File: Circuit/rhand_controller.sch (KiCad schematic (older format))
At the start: 25 parts, among them P1 RU_ADC, P11 RW_ADC, P2 LU_ADC, P3 RV_ADC, P4 LV_ADC, P5 RW_ADC, P6 LW_ADC, P7 BLUETOOTH, P9 LW_ADC, SW1 EmSW, SW2 SWITCH_INV, U1 STM32F042, U2 IM315TX

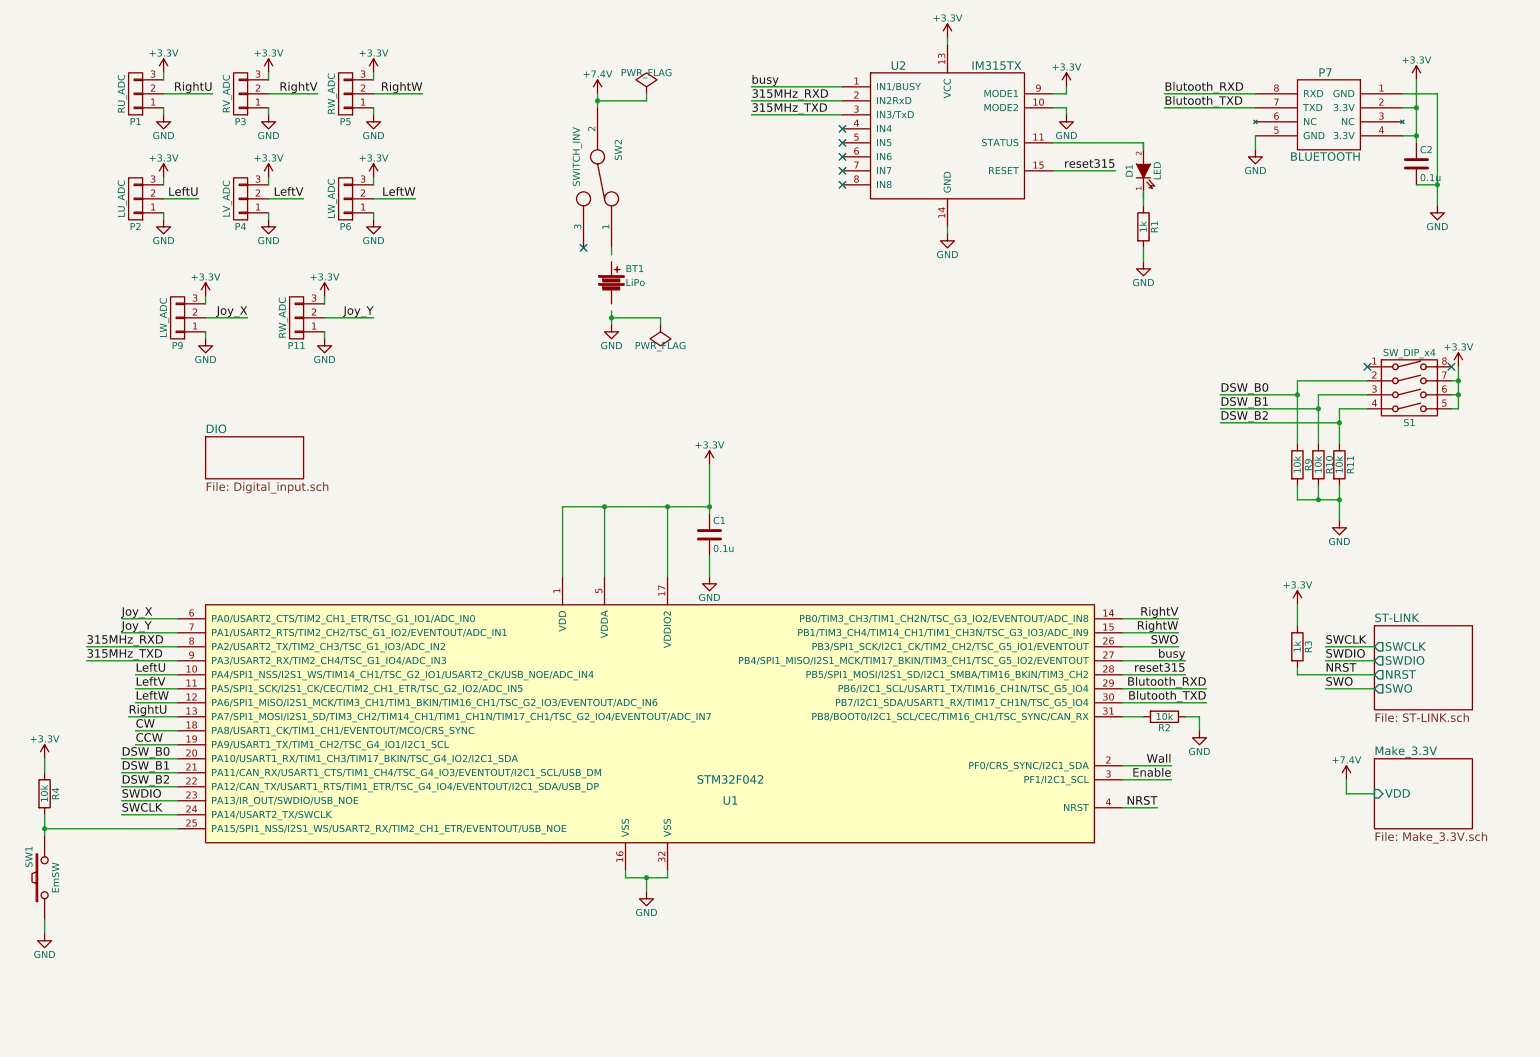
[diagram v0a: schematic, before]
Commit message: シート分けと移動
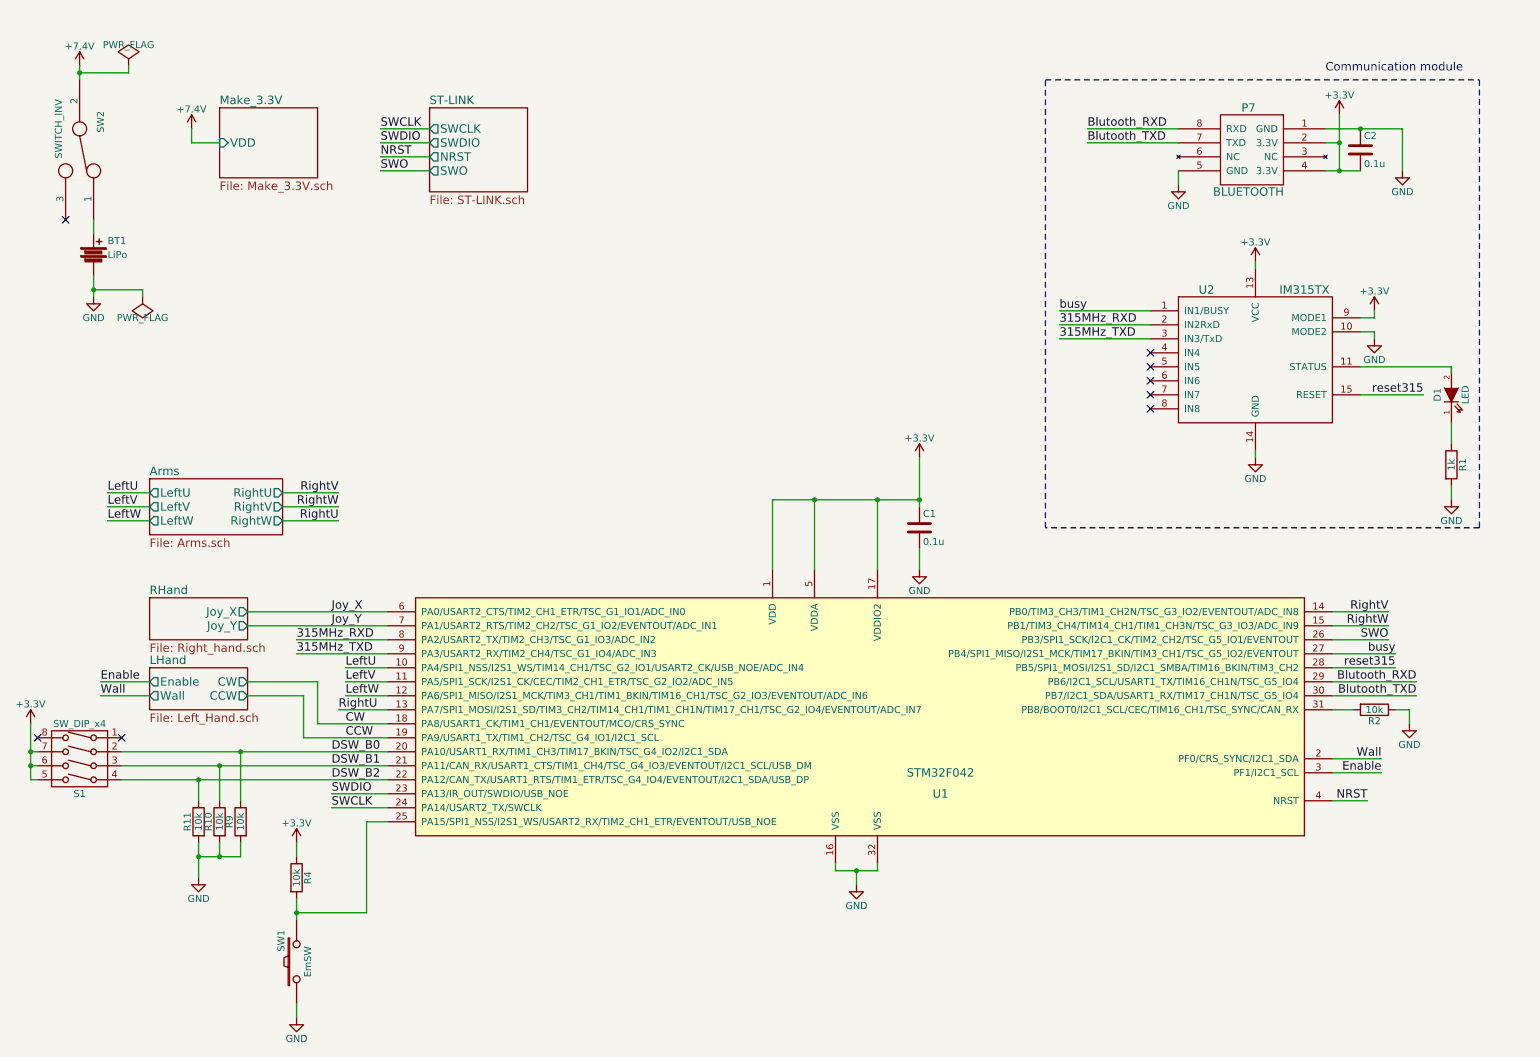
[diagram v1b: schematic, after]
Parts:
- removed P1: RU_ADC, symbol CONN_01X03
- removed P11, P5: RW_ADC, symbol CONN_01X03
- removed P2: LU_ADC, symbol CONN_01X03
- removed P3: RV_ADC, symbol CONN_01X03
- removed P4: LV_ADC, symbol CONN_01X03
- removed P6, P9: LW_ADC, symbol CONN_01X03
- removed R3: 1k, Resistors_SMD:R_0603_HandSoldering, symbol R
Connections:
- net +3V3: now also C2.2; no longer C2.1
- net GND: now also BT1.2, C2.1; no longer C2.2
- net at BT1.1: now also SW2.1
- net at D1.1 (K): now also R1.1
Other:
- note added: "Communication module"
- moved on the sheet: BT1, C1, C2, D1, P7, R1, R10, R11, R2, R4, R9, S1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
